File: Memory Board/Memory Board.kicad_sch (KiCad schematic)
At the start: 37 parts, among them IC1 W25Q01JVZEIQ, IC2 MCP2557FDT-H_MNY, J1 USB4056-03-A_REVA2, J2 Conn_01x04_Socket, J3 Conn_01x04_Socket, J4 Conn_01x04_Socket, SW1 SW_SPST, SW2 SW_SPDT, U1 STM32G473CBTx, U2 LD1117S33TR_SOT223, X1 ECS-2520MV-xxx-xx

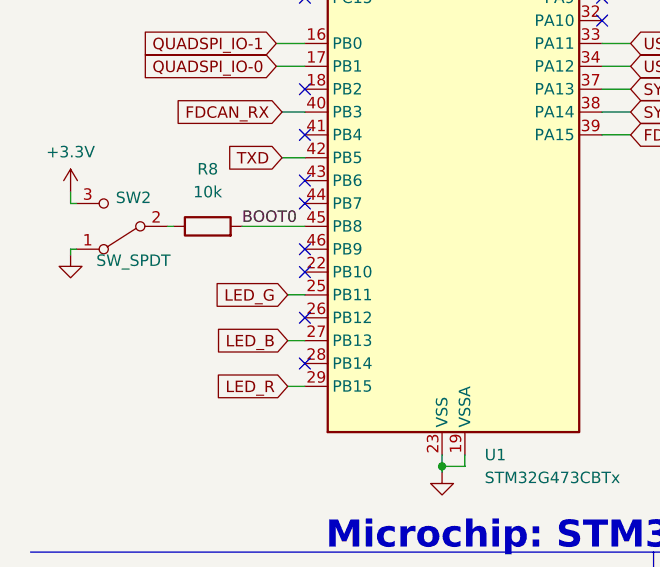
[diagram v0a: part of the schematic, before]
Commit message: Quick fixes
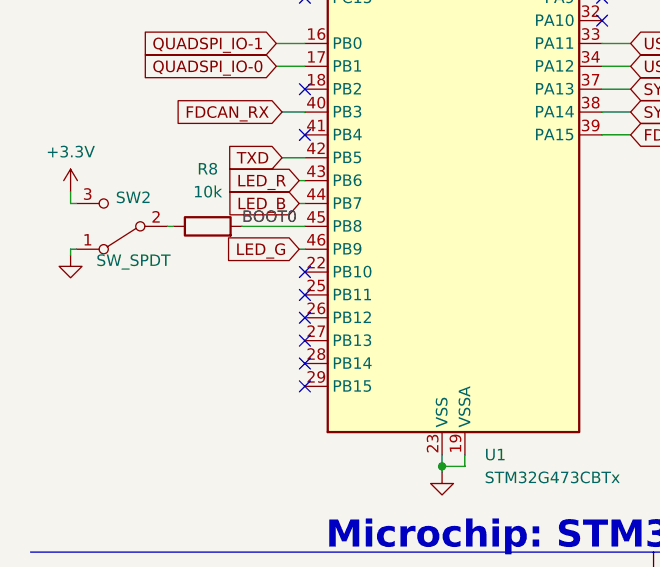
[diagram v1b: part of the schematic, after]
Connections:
- net LED_B: now also U1.44 (PB7); no longer U1.27 (PB13)
- net LED_G: now also U1.46 (PB9); no longer U1.25 (PB11)
- net LED_R: now also U1.43 (PB6); no longer U1.29 (PB15)
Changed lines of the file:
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@@
   (no_connect (at 260.985 139.7))
   (no_connect (at 260.985 129.54))
+  (no_connect (at 42.545 91.44))
   (no_connect (at 42.545 30.48))
   (no_connect (at 260.985 142.24))
@@
   (no_connect (at 42.545 48.26))
   (no_connect (at 42.545 43.18))
-  (no_connect (at 42.545 76.2))
   (no_connect (at 225.425 132.08))
   (no_connect (at 42.545 58.42))
@@
   (no_connect (at 42.545 63.5))
   (no_connect (at 260.985 144.78))
-  (no_connect (at 42.545 71.12))
+  (no_connect (at 42.545 81.28))
   (no_connect (at 225.425 127))
   (no_connect (at 75.565 50.8))
   (no_connect (at 260.985 127))
-  (no_connect (at 42.545 68.58))
   (no_connect (at 260.985 132.08))
+  (no_connect (at 42.545 86.36))
   (no_connect (at 75.565 48.26))
   (no_connect (at 225.425 144.78))
@@
     (stroke (width 0) (type default))
   )
+  (wire (pts (xy 41.91 71.12) (xy 42.545 71.12))
+    (stroke (width 0) (type default))
+  )
   (wire (pts (xy 122.555 184.785) (xy 123.19 184.785))
     (stroke (width 0) (type default))
@@
     (stroke (width 0) (type default))
   )
-  (wire (pts (xy 40.64 81.28) (xy 42.545 81.28))
-    (stroke (width 0) (type default))
-  )
   (wire (pts (xy 211.455 66.04) (xy 208.28 66.04))
     (stroke (width 0) (type default))
@@
     (stroke (width 0) (type default))
   )
-  (wire (pts (xy 40.64 91.44) (xy 42.545 91.44))
-    (stroke (width 0) (type default))
-  )
   (polyline (pts (xy 185.42 115.57) (xy 208.915 115.57))
     (stroke (width 0) (type default))
@@
     (stroke (width 0) (type default))
   )
+  (wire (pts (xy 41.91 68.58) (xy 42.545 68.58))
+    (stroke (width 0) (type default))
+  )
+  (wire (pts (xy 41.91 76.2) (xy 42.545 76.2))
+    (stroke (width 0) (type default))
+  )
   (wire (pts (xy 262.89 153.67) (xy 262.89 152.4))
     (stroke (width 0) (type default))
@@
   )
   (wire (pts (xy 203.835 18.415) (xy 203.835 19.685))
-    (stroke (width 0) (type default))
-  )
-  (wire (pts (xy 40.64 86.36) (xy 42.545 86.36))
     (stroke (width 0) (type default))
   )
@@
     (effects (font (size 1.27 1.27)) (justify left bottom))
   )
-  (global_label "LED_R" (shape input) (at 40.64 91.44 180) (fields_autoplaced)
-    (effects (font (size 1.27 1.27)) (justify right))
-    (property "Intersheetrefs" "${INTERSHEET_REFS}" (at 31.9701 91.44 0)
+  (global_label "LED_R" (shape input) (at 41.91 68.58 180) (fields_autoplaced)
+    (effects (font (size 1.27 1.27)) (justify right))
+    (property "Intersheetrefs" "${INTERSHEET_REFS}" (at 33.2401 68.58 0)
       (effects (font (size 1.27 1.27)) (justify right) hide)
     )
@@
     )
   )
-  (global_label "LED_B" (shape input) (at 40.64 86.36 180) (fields_autoplaced)
-    (effects (font (size 1.27 1.27)) (justify right))
-    (property "Intersheetrefs" "${INTERSHEET_REFS}" (at 31.9701 86.36 0)
+  (global_label "LED_B" (shape input) (at 41.91 71.12 180) (fields_autoplaced)
+    (effects (font (size 1.27 1.27)) (justify right))
+    (property "Intersheetrefs" "${INTERSHEET_REFS}" (at 33.2401 71.12 0)
       (effects (font (size 1.27 1.27)) (justify right) hide)
     )
@@
     )
   )
-  (global_label "LED_G" (shape input) (at 40.64 81.28 180) (fields_autoplaced)
-    (effects (font (size 1.27 1.27)) (justify right))
-    (property "Intersheetrefs" "${INTERSHEET_REFS}" (at 31.9701 81.28 0)
-      (effects (font (size 1.27 1.27)) (justify right) hide)
-    )
+  (global_label "LED_G" (shape input) (at 41.91 76.2 180) (fields_autoplaced)
+    (effects (font (size 1.27 1.27)) (justify right))
+    (property "Intersheetrefs" "${INTERSHEET_REFS}" (at 33.2401 76.2 0)
+      (effects (font (size 1.27 1.27)) (justify right) hide)
+    )
